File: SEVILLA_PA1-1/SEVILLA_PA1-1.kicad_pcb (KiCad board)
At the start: 2 copper layers, 78 x 61.5 mm, 11 parts, among them SW1 SW_DIP_x05, U1 74LS00, U2 74LS04, U3 74LS10

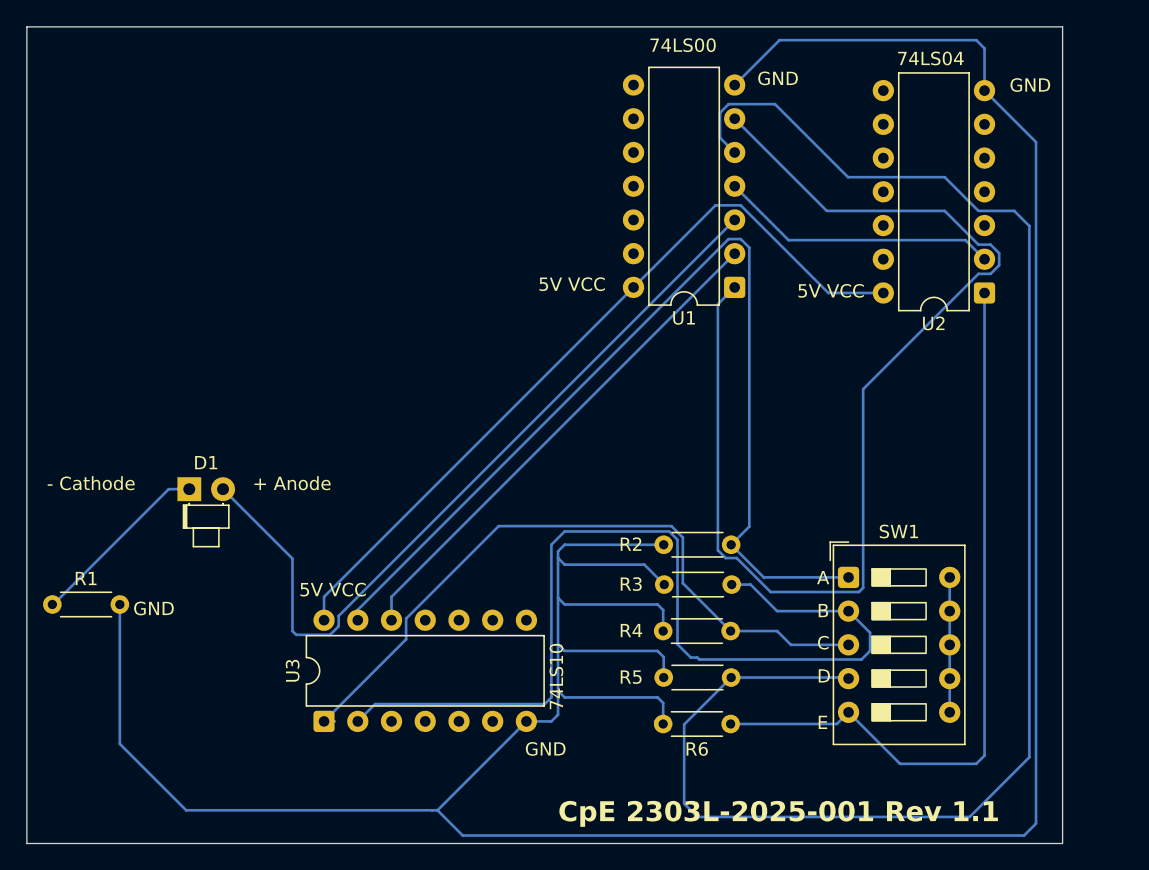
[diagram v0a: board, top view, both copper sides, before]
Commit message: Refactor code structure for improved readability and maintainability
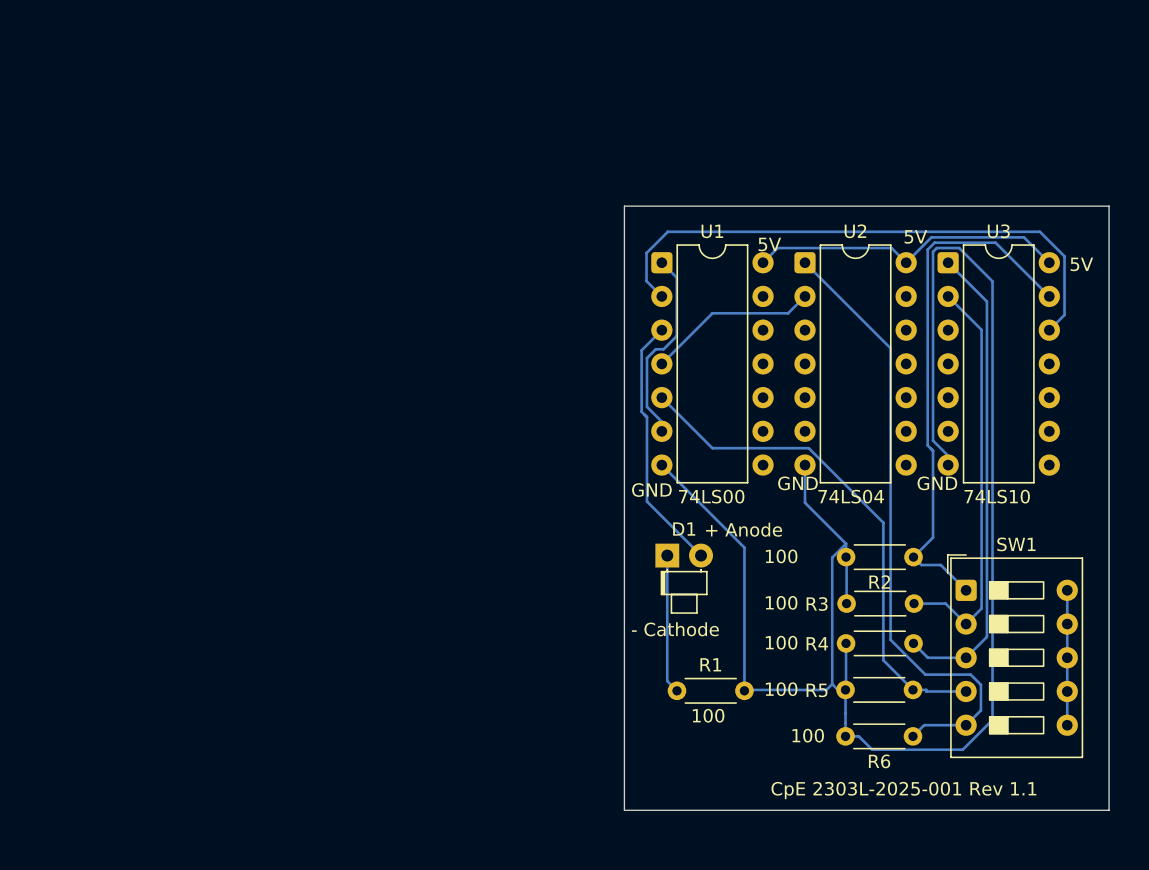
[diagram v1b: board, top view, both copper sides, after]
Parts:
- moved U3 58.3 mm to (159.4, 93.8), turned to 0 degrees
- moved R1 47.5 mm to (139.0, 126.0)
- moved D1 36.3 mm to (138.2, 115.8)
- moved R3 13.8 mm to (156.8, 119.4)
- moved R4 13.8 mm to (156.8, 122.4)
- moved R2 13.8 mm to (156.8, 115.9)
- moved R6 13.8 mm to (156.7, 129.4)
- moved R5 13.7 mm to (156.7, 125.9)
- moved U2 13.7 mm to (148.6, 93.8), turned to 0 degrees
- moved SW1 8.91 mm to (160.7, 118.4)
- moved U1 5.79 mm to (137.8, 93.8), turned to 0 degrees
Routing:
- net GND: track 235.7 -> 125.4 mm
- net Net-(R5-Pad1): track 118.9 -> 38.2 mm
- net Net-(U1-Pad1): track 86.8 -> 14.9 mm
- net Net-(R3-Pad1): track 73.4 -> 30.8 mm
- net Net-(D1-A): track 59.7 -> 19.7 mm
- net +5V: track 58.8 -> 24.1 mm
- net Net-(R2-Pad1): track 74.9 -> 40.2 mm
- net Net-(R4-Pad1): track 53.0 -> 36.0 mm
- net Net-(R6-Pad1): track 56.2 -> 47.1 mm
- net Net-(U1-Pad4): track 21.1 -> 12.9 mm
- net Net-(U1-Pad2): track 38.3 -> 42.7 mm
- net Net-(D1-K): track 14.4 -> 10.5 mm
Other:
- board size 78 x 61.5 mm -> 36.5 x 45.5 mm
- board text added: "100"
- board text added: "5V"
- board text removed: "5V VCC"
- board text removed: "A"
- board text removed: "B"
- board text removed: "C"
- board text removed: "D"
- board text removed: "E"
